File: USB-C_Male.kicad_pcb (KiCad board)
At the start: 2 copper layers, 8.2 x 5 mm, 4 parts, among them J1 USB_C_Receptacle_PowerOnly_6P, J2 VBUS, J3 CC, J4 GND

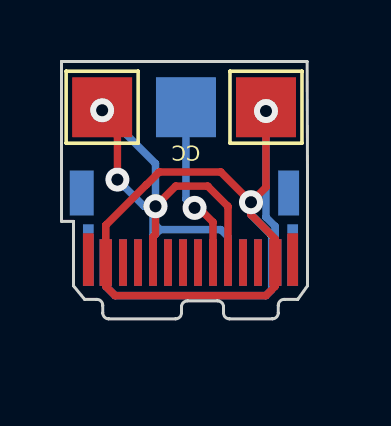
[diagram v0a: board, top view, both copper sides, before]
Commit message: nets and fills
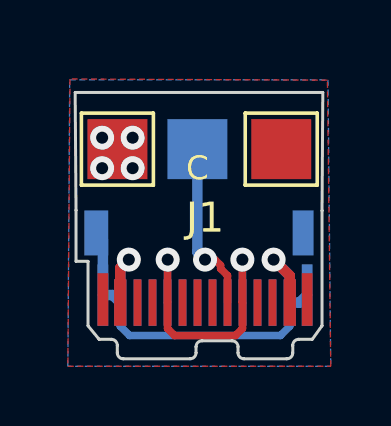
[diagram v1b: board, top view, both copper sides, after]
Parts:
- J2: value VBUS -> V
- J3: value CC -> C
- J4: value GND -> G
- moved J2 6.13 mm to (114.7, 82.2)
- moved J4 5.15 mm to (109.2, 82.2)
- moved J3 1.45 mm to (111.9, 82.2)
- moved J1 1.42 mm to (112.1, 86.1)
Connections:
- net Net-(J1-CC) renamed CC
- net Net-(J2-Pin_1) renamed VBUS
- J1 pad A1: Net-(J4-Pin_1) -> GND
- J1 pad A12: Net-(J4-Pin_1) -> GND
- J1 pad B1: Net-(J4-Pin_1) -> GND
- J1 pad B12: Net-(J4-Pin_1) -> GND
- J1 pad S1: unconnected-(J1-SHIELD-PadS1) -> GND
- J4 pad 1: Net-(J4-Pin_1) -> GND
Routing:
- net Net-(J4-Pin_1): track 37.2 -> 0.00 mm, vias 2 -> 0
- net GND: track 0.00 -> 17.4 mm, vias 0 -> 6
- net VBUS: track 21.3 -> 10.2 mm, vias 3 -> 2
- added copper zone on B.Cu, net GND
- added copper zone on F.Cu, net VBUS
